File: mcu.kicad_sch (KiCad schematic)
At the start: 46 parts, among them CN100 HX JN1.27-2X5 TP H4.9, J100 DM3CS-SF, U100 SW_RUN, U101 STM32F405RGTx, X100 X1E000210127000G

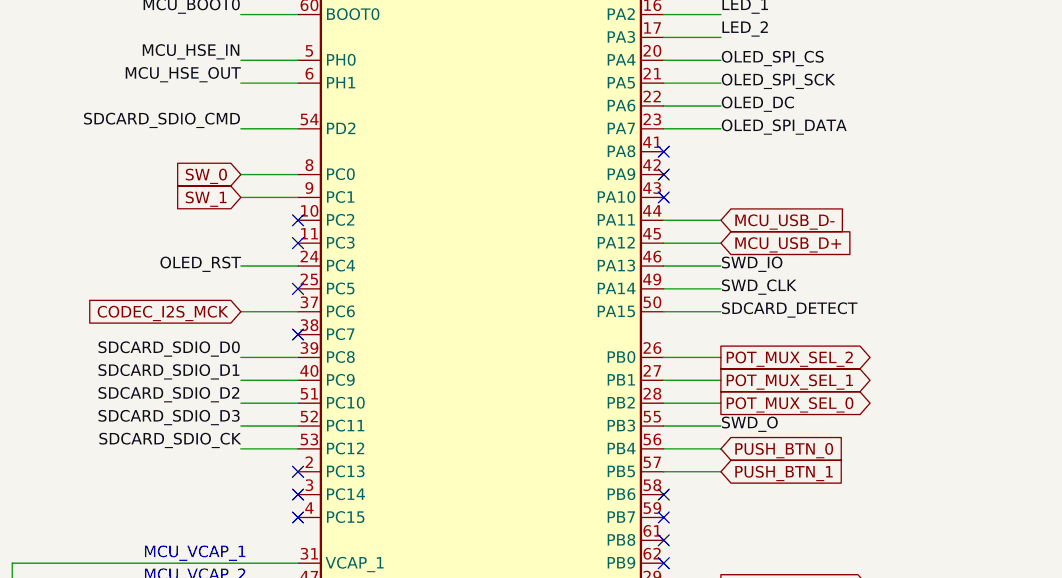
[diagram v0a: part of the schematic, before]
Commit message: last update
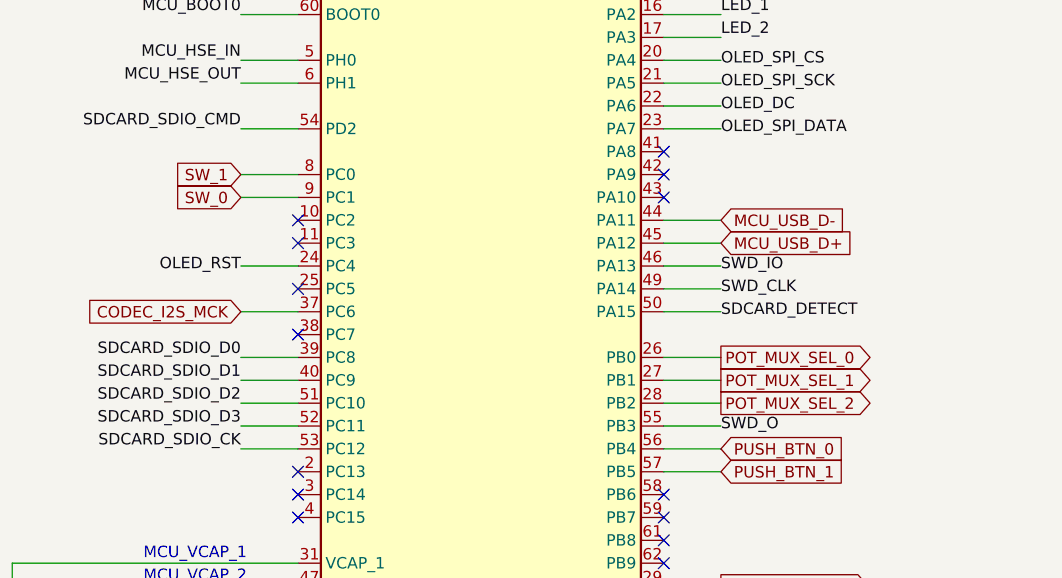
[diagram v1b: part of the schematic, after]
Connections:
- net POT_MUX_SEL_0: now also U101.26 (PB0); no longer U101.28 (PB2)
- net POT_MUX_SEL_2: now also U101.28 (PB2); no longer U101.26 (PB0)
- net SW_0: now also U101.9 (PC1); no longer U101.8 (PC0)
- net SW_1: now also U101.8 (PC0); no longer U101.9 (PC1)
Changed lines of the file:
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@@
 		)
 	)
-	(global_label "SW_0"
+	(global_label "SW_1"
 		(shape input)
 		(at 187.96 76.2 180)
@@
 		)
 	)
-	(global_label "POT_MUX_SEL_2"
+	(global_label "POT_MUX_SEL_0"
 		(shape output)
 		(at 241.3 96.52 0)
@@
 		)
 	)
-	(global_label "SW_1"
+	(global_label "SW_0"
 		(shape input)
 		(at 187.96 78.74 180)
@@
 		)
 	)
-	(global_label "POT_MUX_SEL_0"
+	(global_label "POT_MUX_SEL_2"
 		(shape output)
 		(at 241.3 101.6 0)
